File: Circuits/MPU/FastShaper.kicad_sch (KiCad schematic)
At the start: 34 parts, among them U20 ADA4805-2ARMZ, U21 ADA4805-2ARMZ

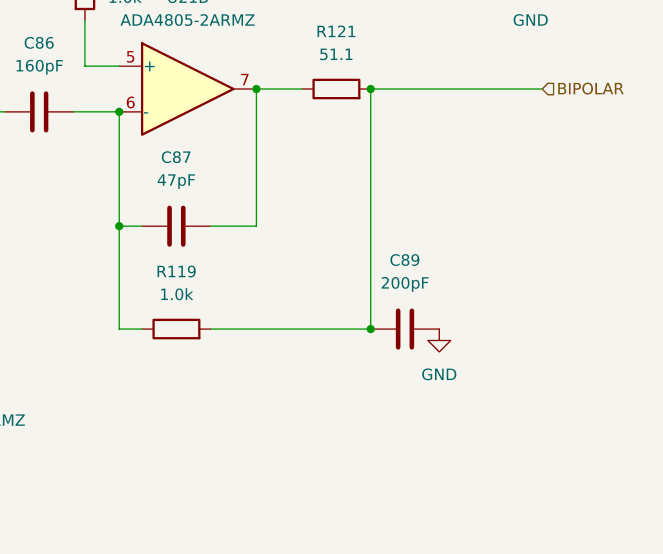
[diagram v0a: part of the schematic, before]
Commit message: revert cap changes from sim. Don't trust it...
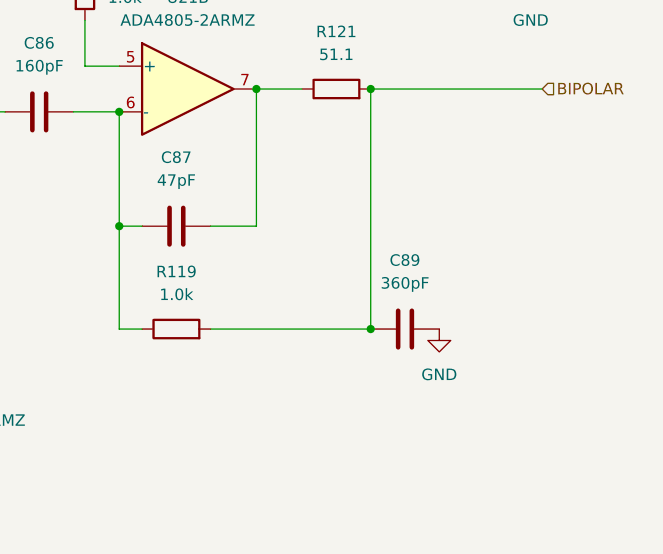
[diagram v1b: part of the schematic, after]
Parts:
- C89: value 200pF -> 360pF
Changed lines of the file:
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@@
 			)
 		)
-		(property "Value" "200pF"
+		(property "Value" "360pF"
 			(at 190.5 127 90)
 			(effects
